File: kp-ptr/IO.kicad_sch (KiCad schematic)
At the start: 10 parts, among them Q5 NMOS_SOT23

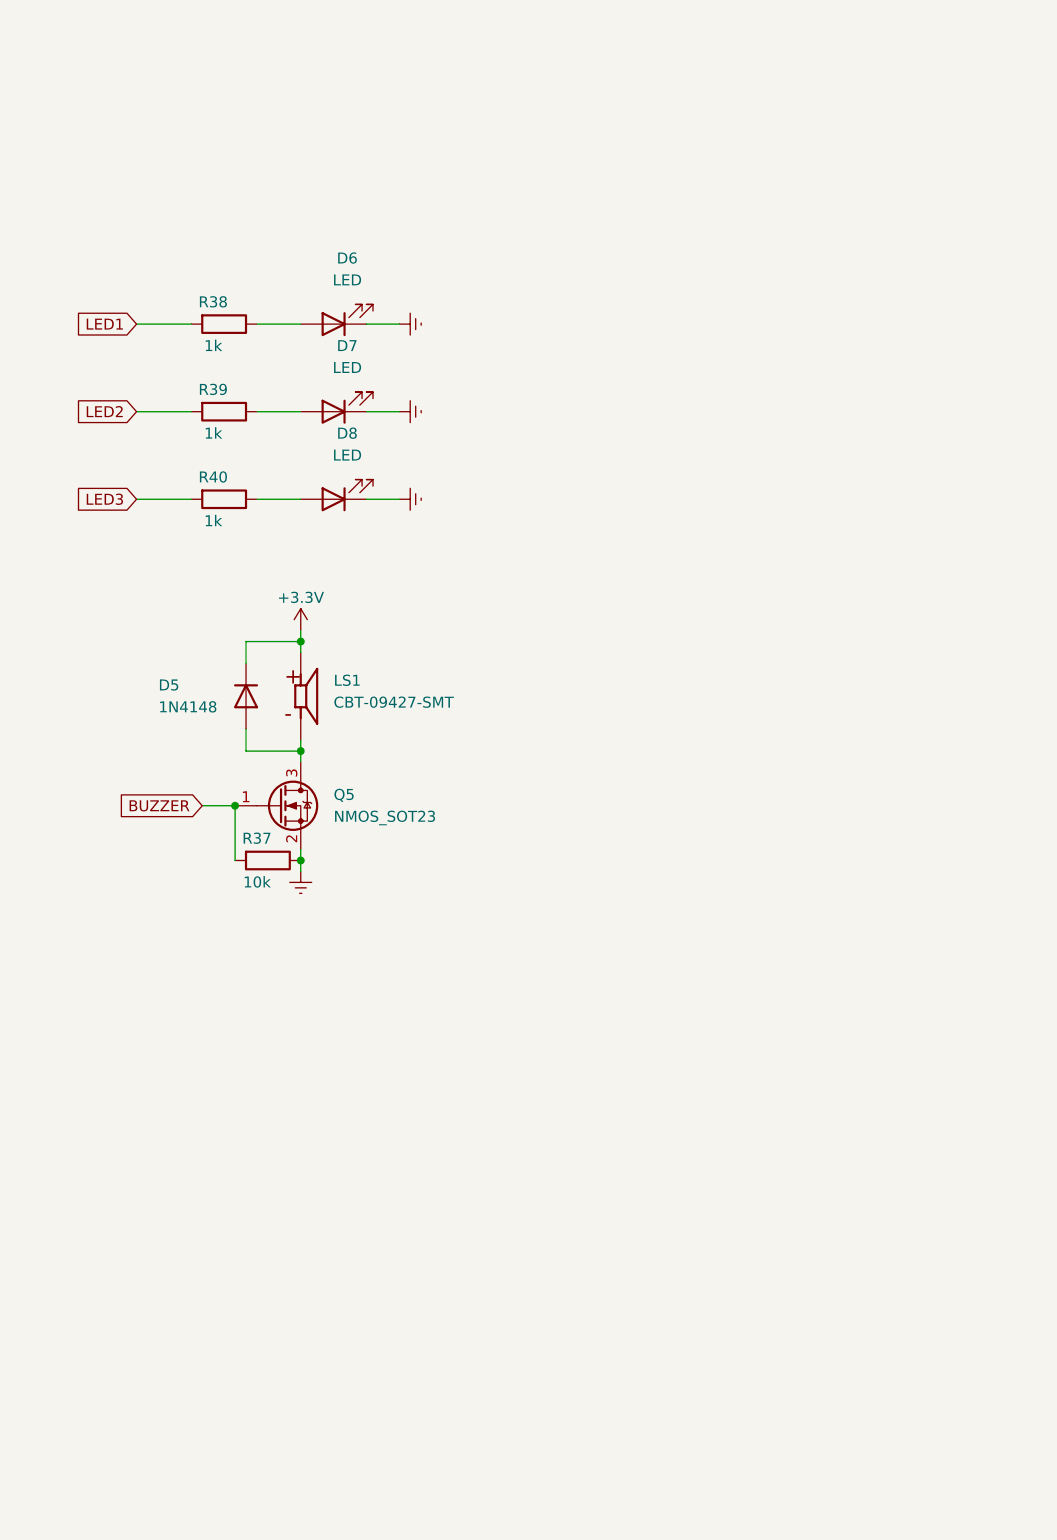
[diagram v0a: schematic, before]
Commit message: Szlifowanie schematu
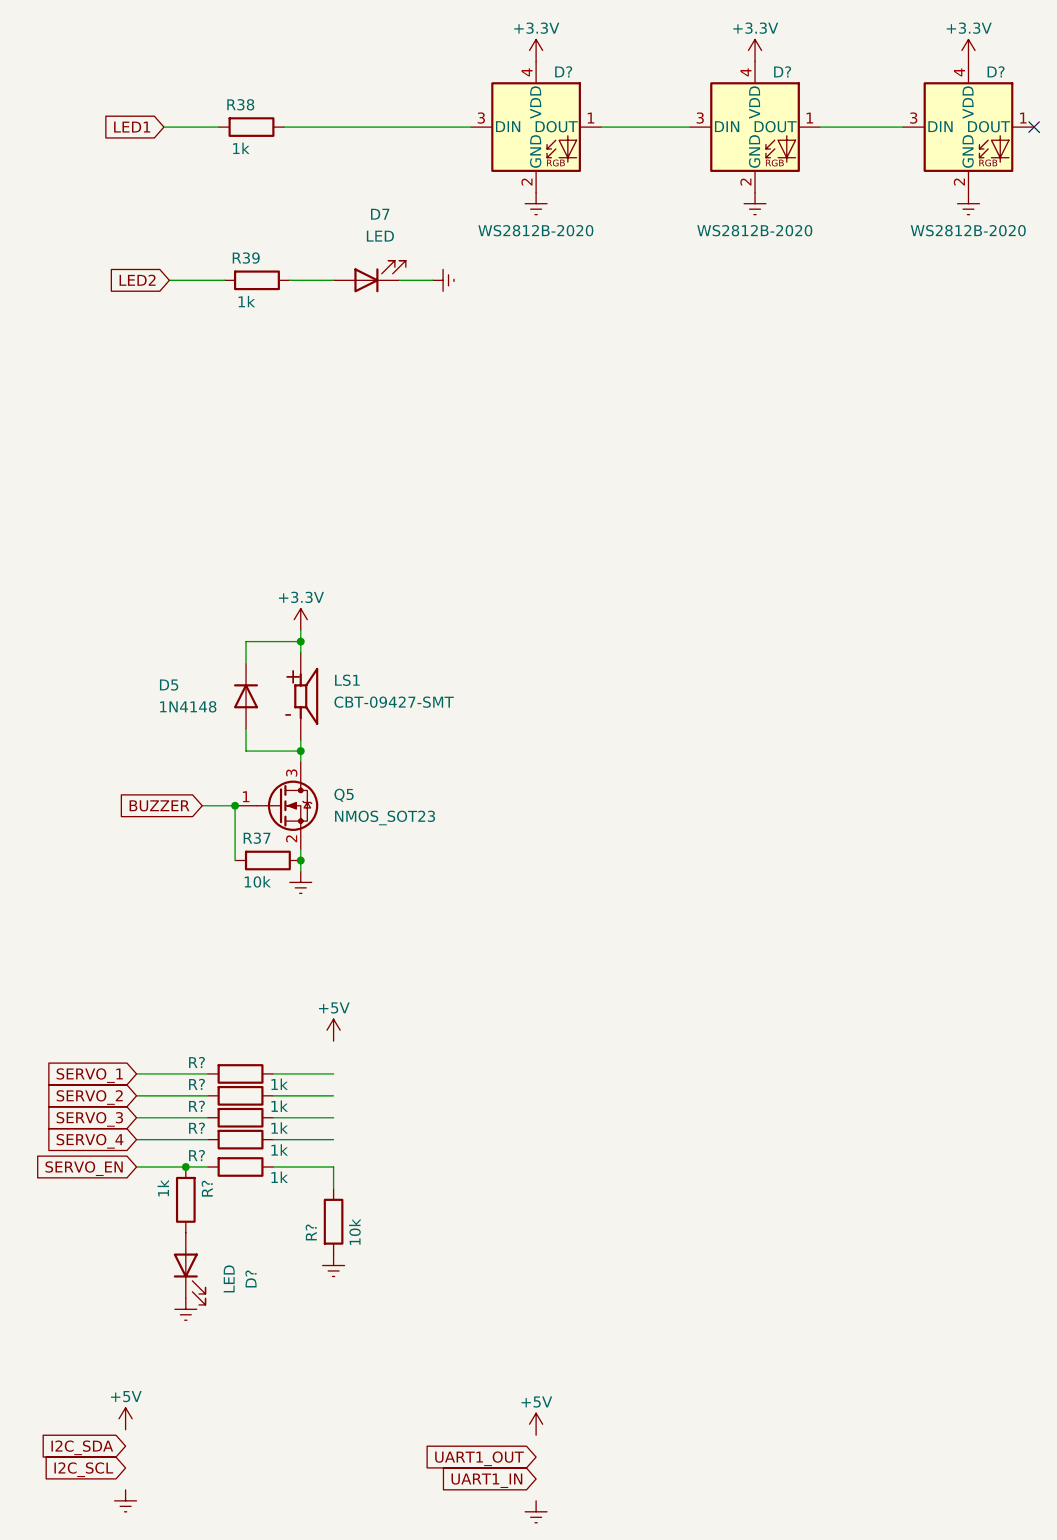
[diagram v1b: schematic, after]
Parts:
- removed D6, D8: LED, LED_SMD:LED_0402_1005Metric_Pad0.77x0.64mm_HandSolder, symbol Device:LED
- removed R40: 1k, Resistor_SMD:R_0402_1005Metric_Pad0.72x0.64mm_HandSolder, symbol Device:R
- added D? (x3): WS2812B-2020, symbol KP-PTR_lib:WS2812B-2020
- added D?: LED, LED_SMD:LED_0402_1005Metric_Pad0.77x0.64mm_HandSolder, symbol Device:LED
- added R? (x6): 1k, Resistor_SMD:R_0402_1005Metric_Pad0.72x0.64mm_HandSolder, symbol Device:R
- added R?: 10k, Resistor_SMD:R_0402_1005Metric_Pad0.72x0.64mm_HandSolder, symbol Device:R
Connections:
- net +3V3: now also D?.4 (VDD), D?.4 (VDD), D?.4 (VDD)
- net Earth: now also D?.1 (K), D?.2 (GND), D?.2 (GND), D?.2 (GND), R?.2
- net at R38.1: now also D?.3 (DIN)
- new net: D?.1 (DOUT), D?.3 (DIN) (x2)
- new net: D?.2 (A), R?.1
- new net: R?.1, R?.1
- new net SERVO_1: R?.2
- new net SERVO_2: R?.2
- new net SERVO_3: R?.2
- new net SERVO_4: R?.2
- new net SERVO_EN: R?.2, R?.2
- no-connect marks 0 -> 1
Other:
- moved on the sheet: D7, R38, R39
